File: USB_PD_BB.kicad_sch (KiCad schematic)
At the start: 7 parts, among them CN1 53375-0410, CN2 10126-5212PC, CN3 UJC-HP-3-SMT-TR, U3 IP2721D

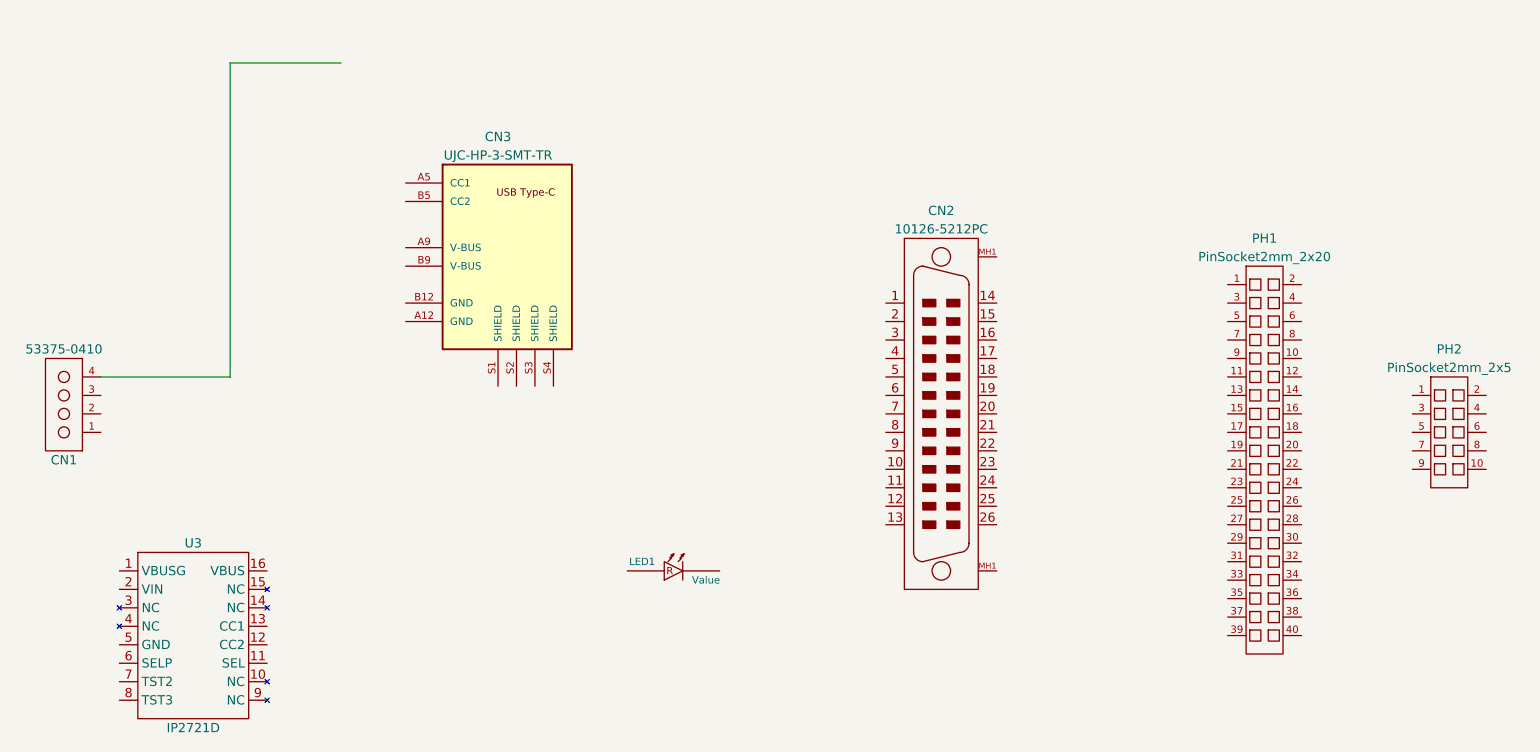
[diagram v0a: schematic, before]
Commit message: add FET ans Switch
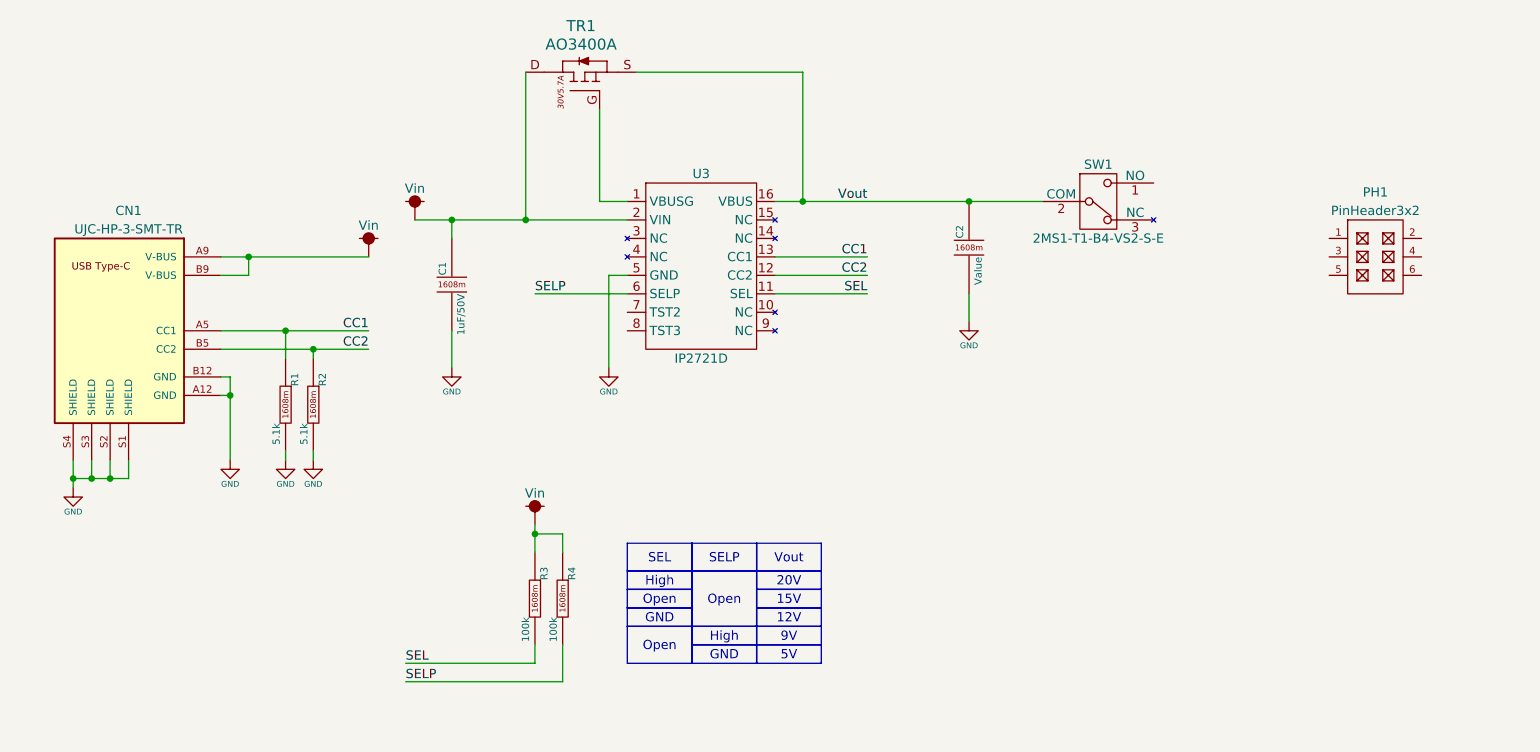
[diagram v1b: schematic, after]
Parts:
- removed CN1: 53375-0410, Connector:53375-0410, symbol Connector:53375-0410
- removed CN2: 10126-5212PC, Connector:10126-5212PC, symbol Connector:10126-5212PC
- removed CN3: UJC-HP-3-SMT-TR, Connector:UJC-HP-3-SMT-TR, symbol Connector:UJC-HP-3-SMT-TR
- removed LED1: Value, Basic:LED1608mRED, symbol Basic:LED1608m_RED
- removed PH1: PinSocket2mm_2x20, PinSocket:PinSocket2mm_2x20, symbol PinSocket:PinSocket2mm_2x20
- removed PH2: PinSocket2mm_2x5, PinSocket:PinSocket2mm_2x5, symbol PinSocket:PinSocket2mm_2x5
- added C1: 1uF/50V, Basic:CAP1608m, symbol Basic:C1608m
- added C2: Value, Basic:CAP1608m, symbol Basic:C1608m
- added CN1: UJC-HP-3-SMT-TR, Connector:UJC-HP-3-SMT-TR, symbol Connector:UJC-HP-3-SMT-TR
- added PH1: PinHeader3x2, PinHeader:PinHeader3x2, symbol PinHeader:PinHeader3x2
- added R1, R2: 5.1k, Basic:REG1608m, symbol Basic:R1608m
- added R3, R4: 100k, Basic:REG1608m, symbol Basic:R1608m
- added SW1: 2MS1-T1-B4-VS2-S-E, Switch:2MS1-T1-B4-VS2-Q-E-S, symbol Switch:2MS1-T1-B4-VS2-Q-E-S
- added TR1: AO3400A, Discrete:AO3400A, symbol Discrete:AO3400A
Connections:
- net at U3.1 (VBUSG): now also TR1.G
- net SEL: now reaches U3.11 (SEL)
- net SEL: now also R3.2
- net CC2: now reaches U3.12 (CC2)
- net CC2: now also CN1.B5 (CC2), R2.1
- net CC1: now reaches U3.13 (CC1)
- net CC1: now also CN1.A5 (CC1), R1.1
- net Vout: now reaches U3.16 (VBUS)
- net Vout: now also C2.1, SW1.2 (COM), TR1.S
- net Vin: now reaches U3.2 (VIN)
- net Vin: now also C1.1, CN1.A9 (V-BUS), CN1.B9 (V-BUS), R3.1, R4.1, TR1.D
- net GND: now reaches U3.5 (GND)
- net GND: now also C1.2, C2.2, CN1.A12 (GND), CN1.B12 (GND), CN1.S1 (SHIELD), CN1.S2 (SHIELD), CN1.S3 (SHIELD), CN1.S4 (SHIELD), R1.2, R2.2
- net SELP: now reaches U3.6 (SELP)
- net SELP: now also R4.2
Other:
- moved on the sheet: U3
